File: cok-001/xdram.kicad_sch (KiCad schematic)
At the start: 38 parts, among them U1201 Y0_XDR0, U1202 Y0_XDR1, U1301 Y1_XDR0, U1302 Y1_XDR1

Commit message: seperate out
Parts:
- added C1343, C1344, C1345, C1346, C1347, C1348, C1349, C1350, C1351, C1352, C1353, C1354, C1355, C1356, C1357, C1358, C1359, C1360, C1361, C1362, C1363, C1364, C1365, C1366, C1367, C1368, C1369, C1370: 0.1u 10V, Capacitor_SMD:C_0402_1005Metric, symbol Device:C
- added C1609, C1610: 1u 10V, Capacitor_SMD:C_0402_1005Metric, symbol Device:C
- added C1611, C1612: 10u 6.3V, Capacitor_SMD:C_0402_1005Metric, symbol Device:C
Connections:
- net +1.2V_YC_RC_VDDIO: now also C1345.1, C1348.1, C1351.1, C1354.1, C1357.1, C1360.1, C1363.1, C1366.1, C1369.1, C1370.1, C1610.1, C1612.1
- net +1.8V_VDD_MEM: now also C1343.1, C1344.1, C1346.1, C1347.1, C1349.1, C1350.1, C1352.1, C1353.1, C1355.1, C1356.1, C1358.1, C1359.1, C1361.1, C1362.1, C1364.1, C1365.1, C1367.1, C1368.1, C1609.1, C1611.1
- net GND: now also C1343.2, C1344.2, C1345.2, C1346.2, C1347.2, C1348.2, C1349.2, C1350.2, C1351.2, C1352.2, C1353.2, C1354.2, C1355.2, C1356.2, C1357.2, C1358.2, C1359.2, C1360.2, C1361.2, C1362.2, C1363.2, C1364.2, C1365.2, C1366.2, C1367.2, C1368.2, C1369.2, C1370.2, C1609.2, C1610.2, C1611.2, C1612.2
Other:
- moved on the sheet: C1313, C1314, C1316, C1317, C1318, C1319, C1320, C1322, C1323, C1324, C1325, C1326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

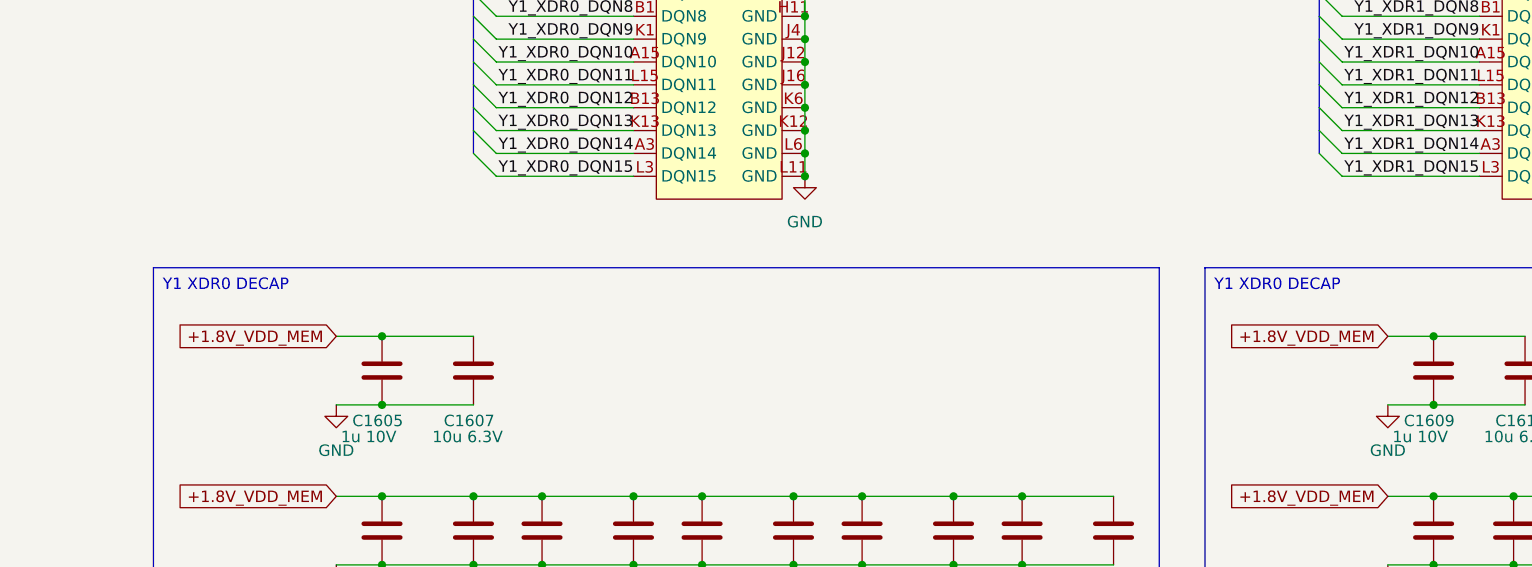
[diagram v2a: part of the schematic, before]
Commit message: update to 9
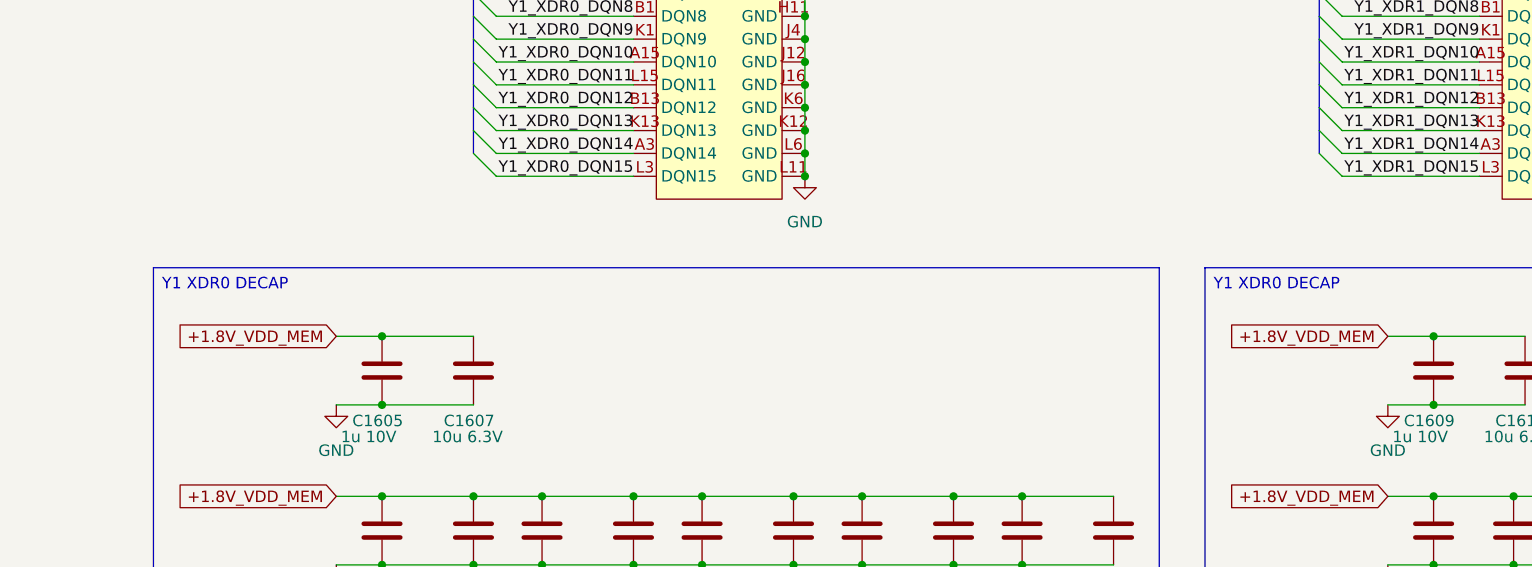
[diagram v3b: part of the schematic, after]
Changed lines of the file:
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@@
 (kicad_sch
-	(version 20231120)
+	(version 20250114)
 	(generator "eeschema")
-	(generator_version "8.0")
+	(generator_version "9.0")
 	(paper "A3")
+	(text_box "Y1 XDR0 DECAP"
+		(exclude_from_sim no)
+		(at 309.88 185.42 0)
+		(size 111.76 85.09)
+		(margins 0.9525 0.9525 0.9525 0.9525)
+		(stroke
+			(width 0)
+			(type default)
+		)
+		(fill
+			(type none)
+		)
+		(effects
+			(font
+				(size 1.27 1.27)
+			)
+			(justify left top)
+		)
+	)
+	(text_box "Y1 XDR0 DECAP"
+		(exclude_from_sim no)
+		(at 193.04 185.42 0)
+		(size 111.76 85.09)
+		(margins 0.9525 0.9525 0.9525 0.9525)
+		(stroke
+			(width 0)
+			(type default)
+		)
+		(fill
+			(type none)
+		)
+		(effects
+			(font
+				(size 1.27 1.27)
+			)
+			(justify left top)
+		)
+	)
 	(junction
 		(at 72.39 147.32)
@@
 		)
 	)
-	(text_box "Y1 XDR0 DECAP"
-		(exclude_from_sim no)
-		(at 309.88 185.42 0)
-		(size 111.76 85.09)
-		(stroke
-			(width 0)
-			(type default)
-		)
-		(fill
-			(type none)
-		)
-		(effects
-			(font
-				(size 1.27 1.27)
-			)
-			(justify left top)
-		)
-	)
-	(text_box "Y1 XDR0 DECAP"
-		(exclude_from_sim no)
-		(at 193.04 185.42 0)
-		(size 111.76 85.09)
-		(stroke
-			(width 0)
-			(type default)
-		)
-		(fill
-			(type none)
-		)
-		(effects
-			(font
-				(size 1.27 1.27)
-			)
-			(justify left top)
-		)
-	)

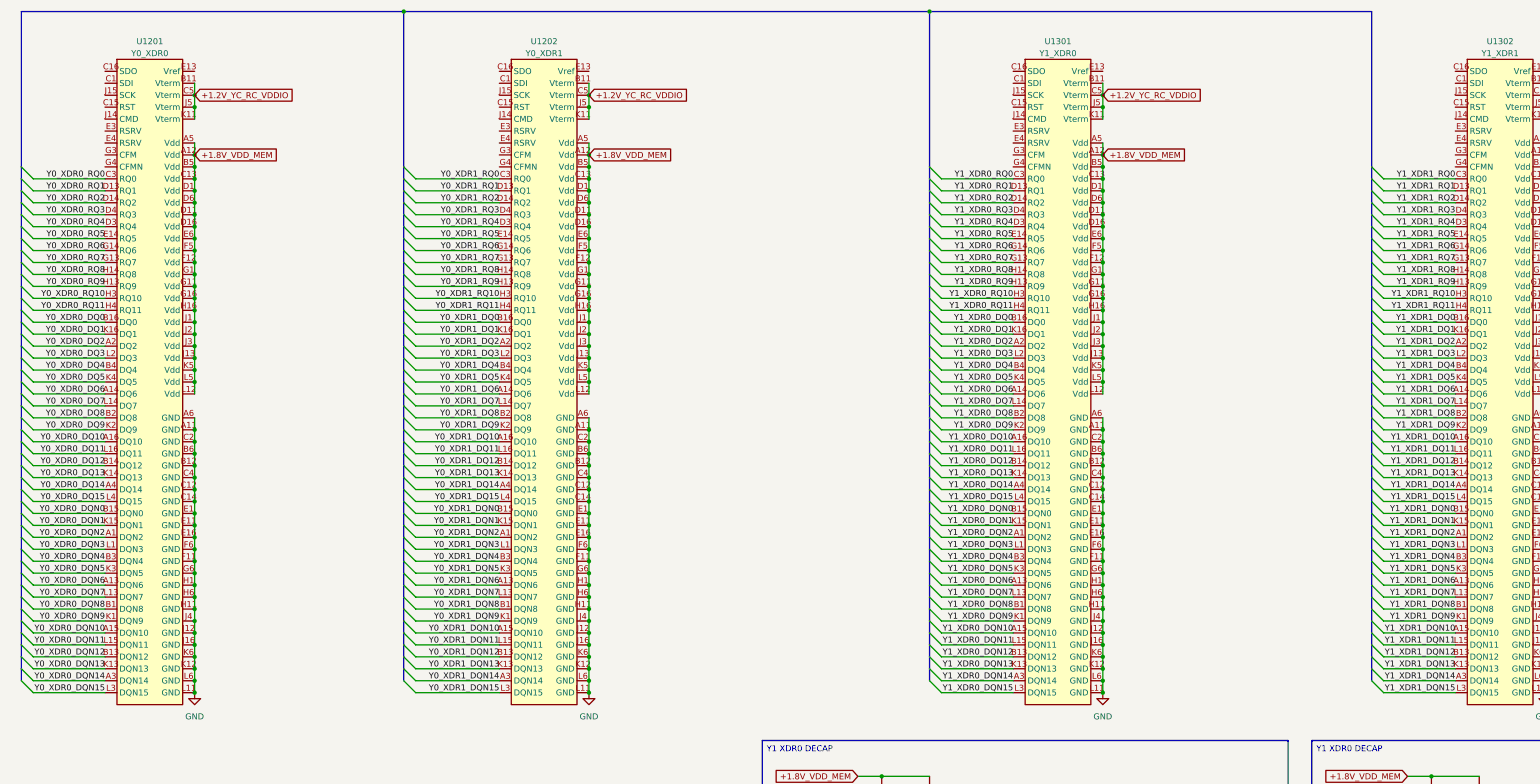
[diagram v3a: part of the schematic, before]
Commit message: cell
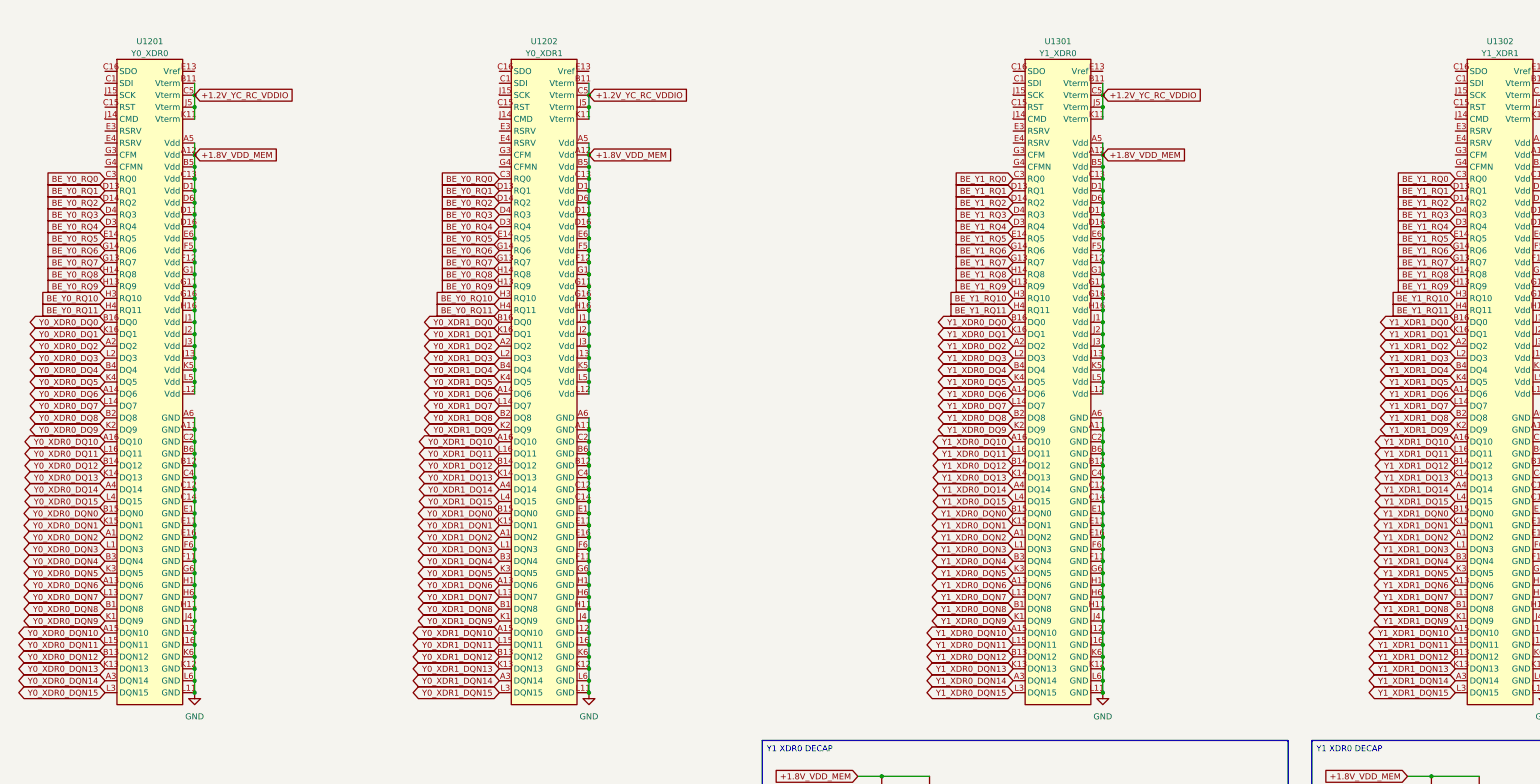
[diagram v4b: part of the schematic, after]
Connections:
- net Y0_XDR1_RQ0 is gone; now on net BE_Y0_RQ0: U1202.C3 (RQ0)
- net Y0_XDR1_RQ1 is gone; now on net BE_Y0_RQ1: U1202.D13 (RQ1)
- net Y0_XDR1_RQ10 is gone; now on net BE_Y0_RQ10: U1202.H3 (RQ10)
- net Y0_XDR1_RQ11 is gone; now on net BE_Y0_RQ11: U1202.H4 (RQ11)
- net Y0_XDR1_RQ2 is gone; now on net BE_Y0_RQ2: U1202.D14 (RQ2)
- net Y0_XDR1_RQ3 is gone; now on net BE_Y0_RQ3: U1202.D4 (RQ3)
- net Y0_XDR1_RQ4 is gone; now on net BE_Y0_RQ4: U1202.D3 (RQ4)
- net Y0_XDR1_RQ5 is gone; now on net BE_Y0_RQ5: U1202.E14 (RQ5)
- net Y0_XDR1_RQ6 is gone; now on net BE_Y0_RQ6: U1202.G14 (RQ6)
- net Y0_XDR1_RQ7 is gone; now on net BE_Y0_RQ7: U1202.G13 (RQ7)
- net Y0_XDR1_RQ8 is gone; now on net BE_Y0_RQ8: U1202.H14 (RQ8)
- net Y0_XDR1_RQ9 is gone; now on net BE_Y0_RQ9: U1202.H13 (RQ9)
- net Y1_XDR1_RQ0 is gone; now on net BE_Y1_RQ0: U1302.C3 (RQ0)
- net Y1_XDR1_RQ1 is gone; now on net BE_Y1_RQ1: U1302.D13 (RQ1)
- net Y1_XDR1_RQ10 is gone; now on net BE_Y1_RQ10: U1302.H3 (RQ10)
- net Y1_XDR1_RQ11 is gone; now on net BE_Y1_RQ11: U1302.H4 (RQ11)
- net Y1_XDR1_RQ2 is gone; now on net BE_Y1_RQ2: U1302.D14 (RQ2)
- net Y1_XDR1_RQ3 is gone; now on net BE_Y1_RQ3: U1302.D4 (RQ3)
- net Y1_XDR1_RQ4 is gone; now on net BE_Y1_RQ4: U1302.D3 (RQ4)
- net Y1_XDR1_RQ5 is gone; now on net BE_Y1_RQ5: U1302.E14 (RQ5)
- net Y1_XDR1_RQ6 is gone; now on net BE_Y1_RQ6: U1302.G14 (RQ6)
- net Y1_XDR1_RQ7 is gone; now on net BE_Y1_RQ7: U1302.G13 (RQ7)
- net Y1_XDR1_RQ8 is gone; now on net BE_Y1_RQ8: U1302.H14 (RQ8)
- net Y1_XDR1_RQ9 is gone; now on net BE_Y1_RQ9: U1302.H13 (RQ9)
- net Y0_XDR0_RQ0 renamed BE_Y0_RQ0
- net Y0_XDR0_RQ1 renamed BE_Y0_RQ1
- net Y0_XDR0_RQ10 renamed BE_Y0_RQ10
- net Y0_XDR0_RQ11 renamed BE_Y0_RQ11
- net Y0_XDR0_RQ2 renamed BE_Y0_RQ2
- net Y0_XDR0_RQ3 renamed BE_Y0_RQ3
- net Y0_XDR0_RQ4 renamed BE_Y0_RQ4
- net Y0_XDR0_RQ5 renamed BE_Y0_RQ5
- net Y0_XDR0_RQ6 renamed BE_Y0_RQ6
- net Y0_XDR0_RQ7 renamed BE_Y0_RQ7
- net Y0_XDR0_RQ8 renamed BE_Y0_RQ8
- net Y0_XDR0_RQ9 renamed BE_Y0_RQ9
- net Y1_XDR0_RQ0 renamed BE_Y1_RQ0
- net Y1_XDR0_RQ1 renamed BE_Y1_RQ1
- net Y1_XDR0_RQ10 renamed BE_Y1_RQ10
- net Y1_XDR0_RQ11 renamed BE_Y1_RQ11
- net Y1_XDR0_RQ2 renamed BE_Y1_RQ2
- net Y1_XDR0_RQ3 renamed BE_Y1_RQ3
- net Y1_XDR0_RQ4 renamed BE_Y1_RQ4
- net Y1_XDR0_RQ5 renamed BE_Y1_RQ5
- net Y1_XDR0_RQ6 renamed BE_Y1_RQ6
- net Y1_XDR0_RQ7 renamed BE_Y1_RQ7
- net Y1_XDR0_RQ8 renamed BE_Y1_RQ8
- net Y1_XDR0_RQ9 renamed BE_Y1_RQ9
